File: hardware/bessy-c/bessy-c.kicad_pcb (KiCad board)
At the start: 2 copper layers, 91.5 x 134.5 mm, 55 parts, among them J1 rotary_encoder, J10 fan, J11 auger, J2 probe0, J3 probe1, J4 probe2, J5 PTD, J6 igniter, J7 Display, J8 fire_pit, J9 line_in, K1 1462042-7, K2 1462042-7, K3 1462042-7, Q1 BC847, Q2 SCS-1002K, Q3 BC847, Q4 BC847, U1 ProS3, U2 ADS1115IDGS, U3 MCP96xx01x-x-MX, U4 IRM-10-5, U5 NAU7802SGI

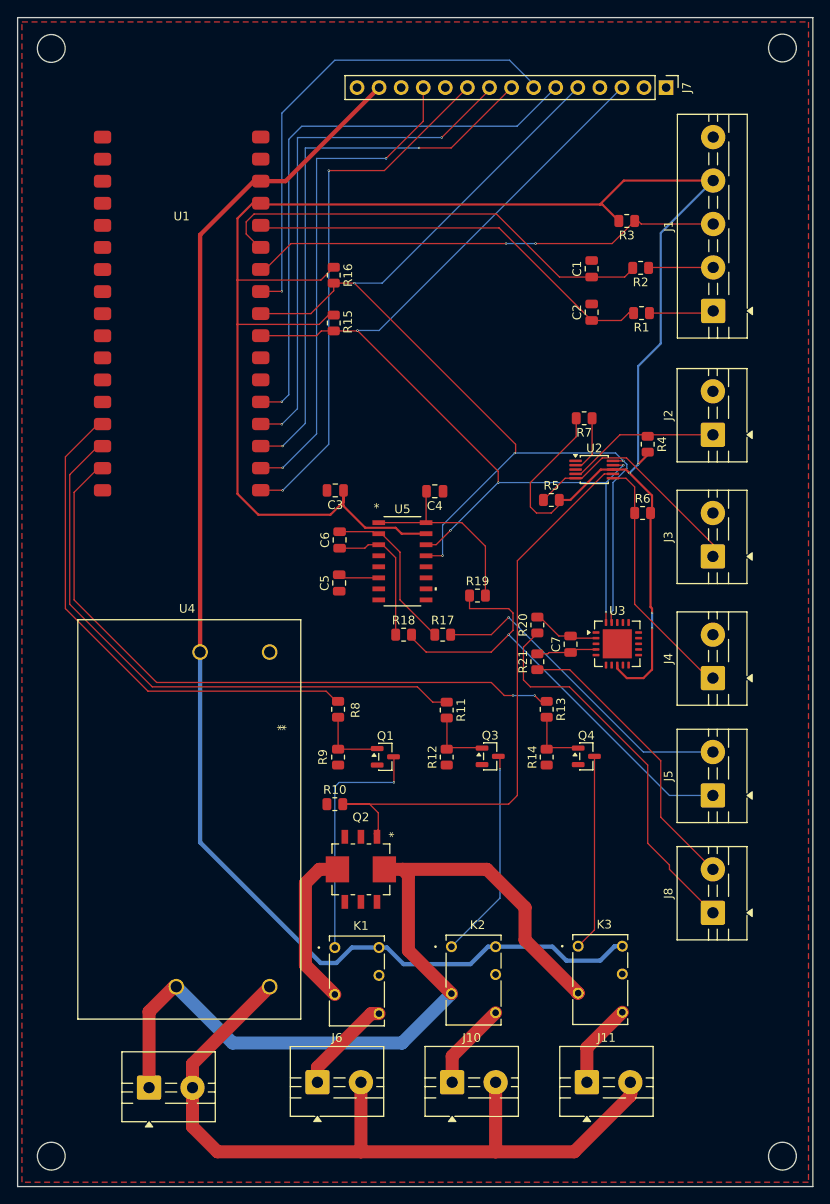
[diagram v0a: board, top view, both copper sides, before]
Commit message: Ordered bessy-c pcba rev 1
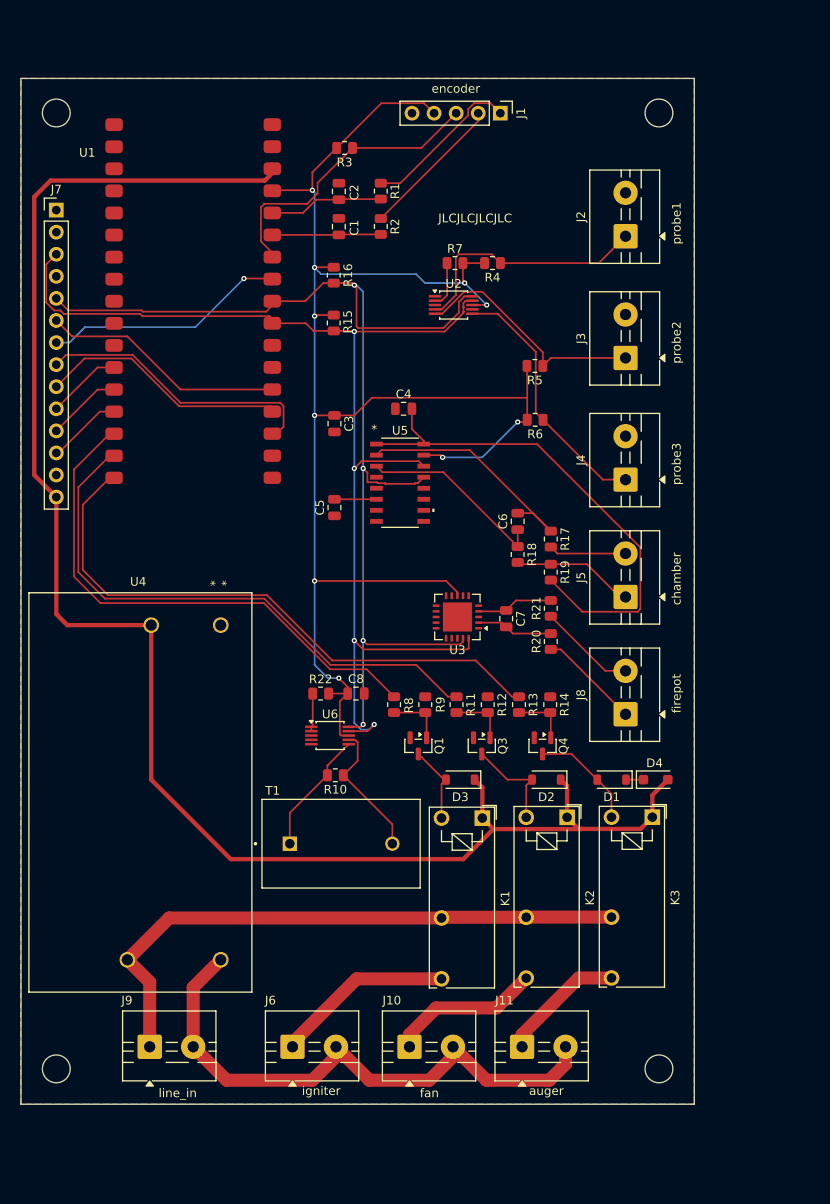
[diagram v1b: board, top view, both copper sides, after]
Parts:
- removed Q2: SCS-1002K, Digikey_SCS_1002K:TRAN_SCS-1002K_SIG
- added C8: 10uF, Capacitor_SMD:C_0805_2012Metric, F.Cu at (94.9, 112.8)
- added D1: 1N4148W, Diode_SMD:D_SOD-123, F.Cu at (124.3, 122.7)
- added D2: 1N4148W, Diode_SMD:D_SOD-123, F.Cu at (116.8, 122.7)
- added D3: 1N4148W, Diode_SMD:D_SOD-123, F.Cu at (106.9, 122.7)
- added D4: BZT52C24, Diode_SMD:D_SOD-123F, F.Cu at (129.4, 122.7)
- added R22: 10k, Resistor_SMD:R_0805_2012Metric, F.Cu at (90.9, 112.8)
- added T1: ZMCT102, kicad-jcl-lib:XFMR_ZMCT102, F.Cu at (93.2, 130.0)
- added U6: ADS1115IDGS, Package_SO:TSSOP-10_3x3mm_P0.5mm, F.Cu at (91.9, 117.6)
- C5, C6, C7: value .1uF -> 0.1uF
- J1: value rotary_encoder -> Conn_01x05; footprint TerminalBlock:TerminalBlock_MaiXu_MX126-5.0-05P_1x05_P5.00mm -> Connector_PinHeader_2.54mm:PinHeader_1x05_P2.54mm_Vertical
- J10: value fan -> DB300V-5.0-2P-BK-S
- J11: value auger -> DB300V-5.0-2P-BK-S
- J2: value probe0 -> DB300V-5.0-2P-BK-S
- J3: value probe1 -> DB300V-5.0-2P-BK-S
- J4: value probe2 -> DB300V-5.0-2P-BK-S
- J5: value PTD -> DB300V-5.0-2P-BK-S
- J6: value igniter -> DB300V-5.0-2P-BK-S
- J7: value Display -> Conn_01x14; footprint Connector_PinHeader_2.54mm:PinHeader_1x15_P2.54mm_Vertical -> Connector_PinHeader_2.54mm:PinHeader_1x14_P2.54mm_Vertical
- J8: value fire_pit -> DB300V-5.0-2P-BK-S
- J9: value line_in -> DB300V-5.0-2P-BK-S
- K1, K2, K3: value 1462042-7 -> G5NB; footprint Digikey_1462042_7_Relay:IM-C_THRU_TEC -> Relay_THT:Relay_SPST_Omron_G5NB
- Q1, Q3, Q4: value BC847 -> MMBT2222A
- R19: value 3k -> 3.3k
- U3: value MCP96xx01x-x-MX -> MCP96L00T-E/MX
- moved J7 71.6 mm to (60.5, 57.1), turned to 0 degrees
- moved R3 33.5 mm to (93.6, 50.0)
- moved J1 33.4 mm to (111.5, 46.0), turned to -90 degrees
- moved R1 33.1 mm to (97.8, 55.0), turned to -90 degrees
- moved C2 32.2 mm to (93.0, 55.0)
- moved R2 30.3 mm to (97.8, 59.0), turned to -90 degrees
- moved C1 29.5 mm to (93.0, 59.0)
- moved R4 27.4 mm to (110.6, 63.2), turned to 180 degrees
- moved J2 25.0 mm to (126.0, 60.2)
- moved J3 25.0 mm to (126.0, 74.2)
- moved J4 25.0 mm to (126.0, 88.2)
- moved J5 25.0 mm to (126.0, 101.7)
- moved J8 25.0 mm to (126.0, 115.2)
- moved U2 24.9 mm to (106.2, 68.1)
- moved R7 23.2 mm to (106.3, 63.2), turned to 0 degrees
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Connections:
- Q1 pad 3: Net-(Q1-C) -> Net-(D3-A)
- Q3 pad 3: Net-(Q3-C) -> Net-(D2-A)
- Q4 pad 3: Net-(Q4-C) -> Net-(D1-A)
- R10 pad 1: GND -> Net-(U6-AIN3)
- R10 pad 2: /igniter_current -> Net-(U6-AIN2)
- U1 pad 16: /tft_cs -> unconnected-(U1-IO13-Pad16)
- U1 pad 17: /tft_dc -> unconnected-(U1-IO12-Pad17)
- U1 pad 18: /IO42 -> /auger
- U1 pad 19: /auger -> /fan
- U1 pad 20: /fan -> /igniter
- U1 pad 21: /igniter -> /tft_cs
- U1 pad 22: /IO38 -> /tft_rst
- U1 pad 23: /IO44 -> /tft_dc
- U2 pad 7: /igniter_current -> unconnected-(U2-AIN3-Pad7)
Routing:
- net /igniter_current: track 69.8 -> 0.00 mm
- net /tft_dc: track 61.0 -> 8.12 mm, vias 2 -> 0
- net +3.3V: track 237.6 -> 187.9 mm, vias 4 -> 10
- net /tft_cs: track 57.3 -> 8.51 mm, vias 2 -> 0
- net /enc_b: track 52.6 -> 12.0 mm
- net Net-(J5-Pin_1): track 53.6 -> 14.1 mm, vias 1 -> 0
- net /spi_miso: track 65.8 -> 28.6 mm, vias 1 -> 0
- net Net-(U5-AVDD/LDO): track 22.7 -> 59.0 mm
- net /enc_a: track 47.3 -> 12.6 mm
- net +5V: track 155.5 -> 189.5 mm
- net Net-(J8-Pin_1): track 44.1 -> 11.7 mm
- net /spi_clk: track 64.2 -> 32.5 mm, vias 2 -> 0
- net /spi_mosi: track 60.5 -> 29.2 mm, vias 2 -> 0
- net Net-(J5-Pin_2): track 37.4 -> 8.92 mm, vias 1 -> 0
- net Net-(Q1-C): track 28.5 -> 0.00 mm, vias 1 -> 0
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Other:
- board size 91.5 x 134.5 mm -> 77.5 x 118 mm
- board text added: "JLCJLCJLCJLC"
- board text removed: "Main Sheet"
